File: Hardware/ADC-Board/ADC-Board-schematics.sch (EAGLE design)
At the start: 27 parts

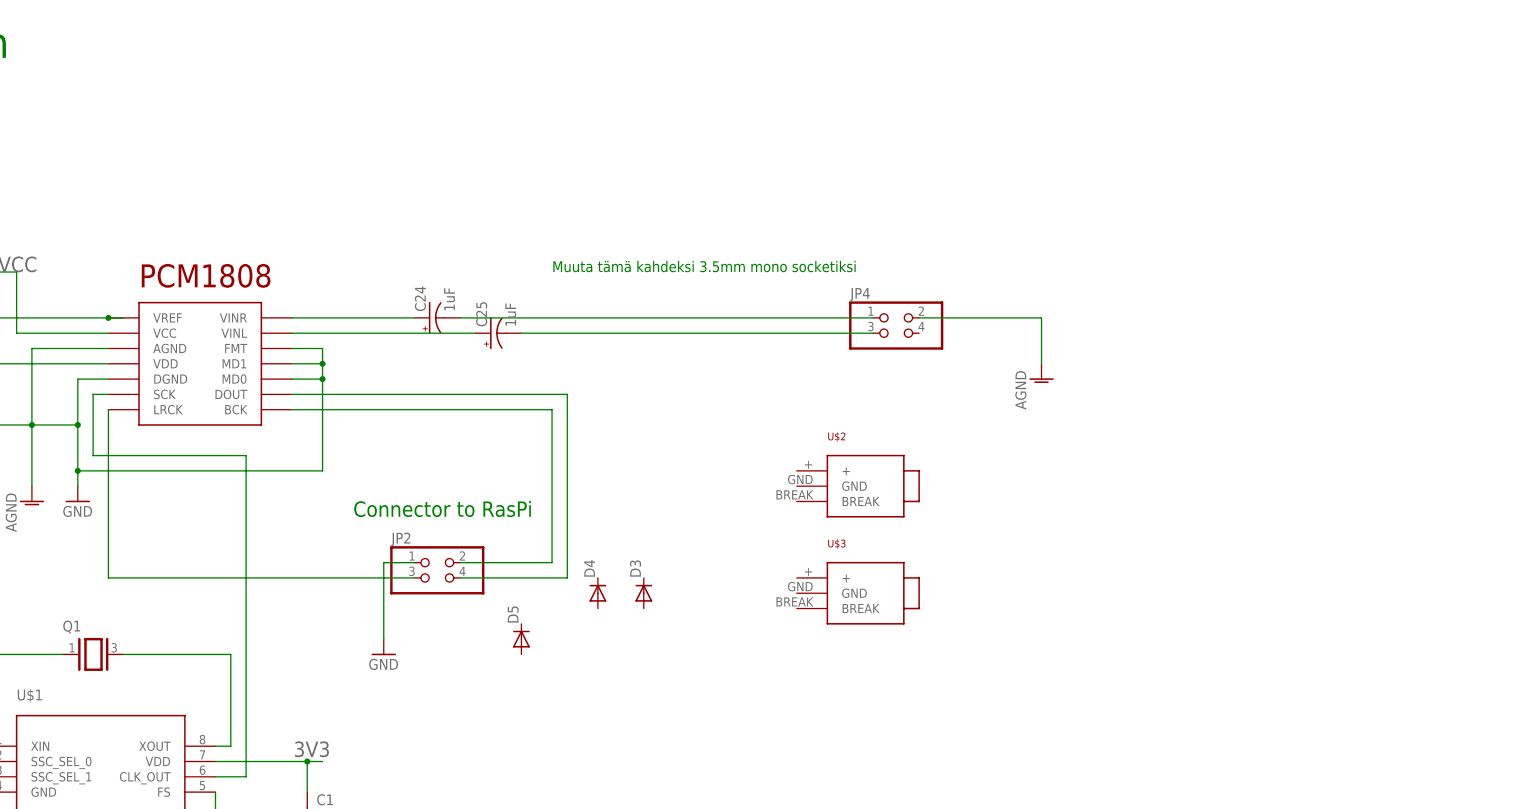
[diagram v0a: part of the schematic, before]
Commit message: some hw changes
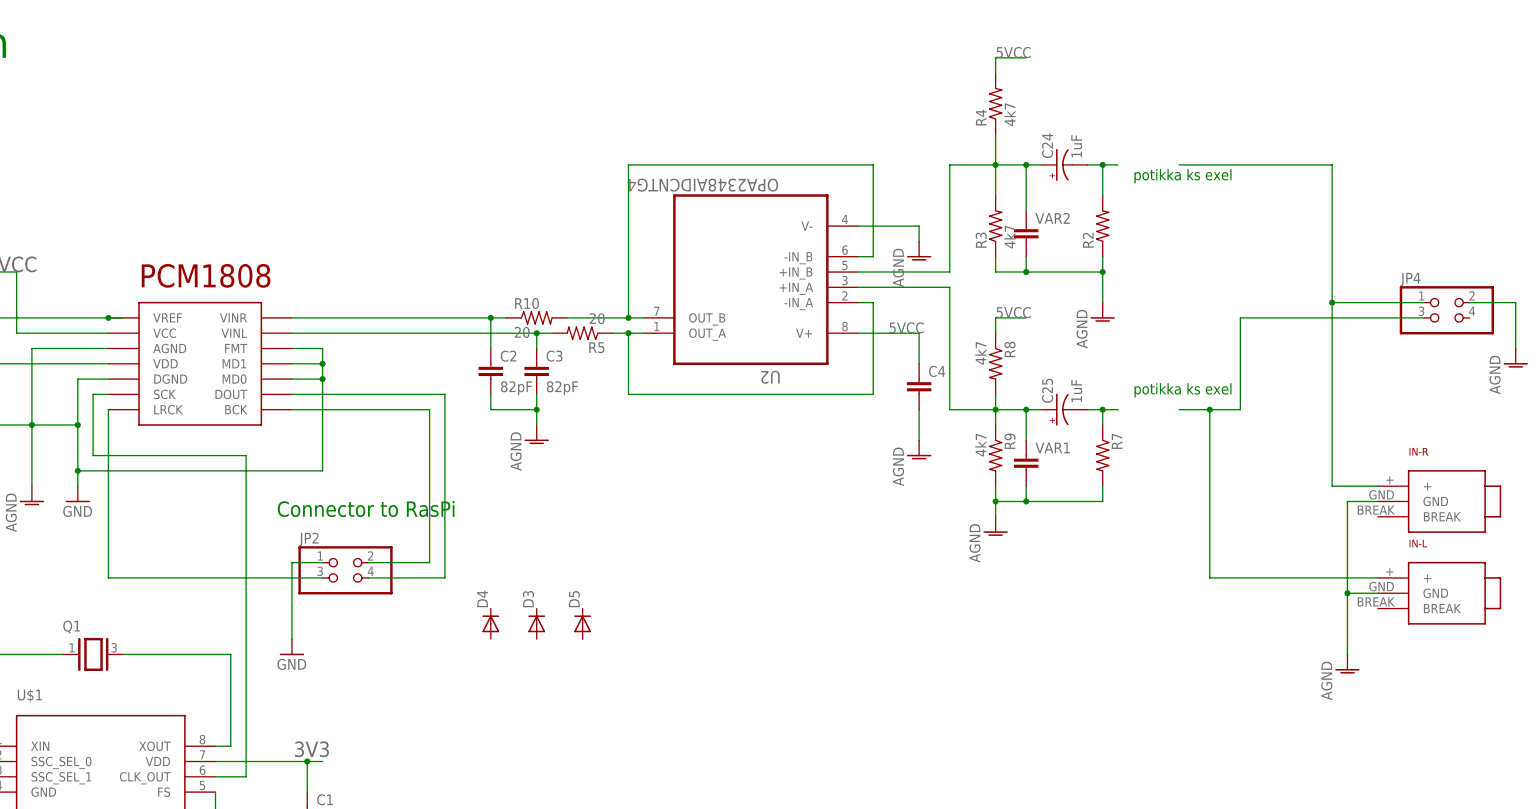
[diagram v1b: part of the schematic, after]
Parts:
- removed U$2, U$3: 3MM5-PLUG, Pekkas_libraries:3MM5-PLUG
- added C2, C3: 82pF, SparkFun-Passives:CAP0603-CAP
- added C4, VAR1, VAR2: (no value), SparkFun-Passives:CAP0603-CAP
- added IN-L, IN-R: 3MM5-PLUG, Pekkas_libraries:3MM5-PLUG
- added R10, R5: 20, SparkFun-Passives:RESISTOR0603-RES
- added R2, R7: (no value), SparkFun-Passives:RESISTOR0603-RES
- added R3, R4, R8, R9: 4k7, SparkFun-Passives:RESISTOR0603-RES
- added U2: OPA2348AIDCNTG4, Pekkas_libraries:OPA2348AIDCNTG4
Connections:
- removed net N$28: C25.+, PCM1808.VINL
- removed net N$36: C24.-, JP4.1
- removed net N$37: C25.-, JP4.3
- new net AGND: C2.2, C3.2, C4.2, IN-L.GND, IN-R.GND, R2.1, R3.1, R7.2, R9.2, U2.V-, VAR1.2, VAR2.2
- new net N$10: R10.2, U2.-IN_B, U2.OUT_B
- new net N$11: C2.1, PCM1808.VINR, R10.1
- new net N$12: IN-R.+, JP4.1
- new net N$13: IN-L.+, JP4.3
- new net N$5: C24.+, R3.2, R4.1, U2.+IN_B, VAR2.1
- new net N$6: R5.1, U2.-IN_A, U2.OUT_A
- new net N$7: C3.1, PCM1808.VINL, R5.2
- new net N$8: C25.-, R7.1
- new net N$9: C25.+, R8.2, R9.1, U2.+IN_A, VAR1.1
- net 5VCC: now also C4.1, R4.2, R8.1, U2.V+
- net N$3: now also C24.-, R2.2; no longer C24.+, PCM1808.VINR
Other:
- note added: "potikka ks exel"
- note removed: "Muuta tämä kahdeksi 3.5mm mono socketiksi"
- moved on the sheet: C24, C25, D3, D4, D5, JP2, JP4
